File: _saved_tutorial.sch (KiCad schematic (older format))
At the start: 239 parts, among them SW0:0 ESC, SW0:1 1, SW0:10 0, SW0:11 -, SW0:12 =, SW0:13 BCKSPC, SW0:14 INS, SW0:15 HOME, SW0:2 2, SW0:3 3, SW0:4 4, SW0:5 5, SW0:6 6, SW0:7 7, SW0:8 8, SW0:9 9, SW1:0 PAGE_UP, SW1:1 TAB, SW1:10 O, SW1:11 P, SW1:12 [, SW1:13 ], SW1:14 \\, SW1:15 DEL, SW1:2 Q, SW1:3 W, SW1:4 E, SW1:5 R, SW1:6 T, SW1:7 Y, SW1:8 U, SW1:9 I, SW2:0 END, SW2:1 PAGE_DOWN, SW2:10 K, SW2:11 L, SW2:12 ;, SW2:13 `, SW2:14 ENTER, SW2:15 LEFT, SW2:2 CAPSLOCK, SW2:3 A, SW2:4 S, SW2:5 D, SW2:6 F, SW2:7 G, SW2:8 H, SW2:9 J, SW3:0 RIGHT, SW3:1 L_SHIFT, SW3:10 ., SW3:11 /, SW3:12 R_SHIFT, SW3:13 UP, SW3:14 DOWN, SW3:15 L_CTRL, SW3:2 Z, SW3:3 X, SW3:4 C, SW3:5 V, SW3:6 B, SW3:7 N, SW3:8 M, SW3:9 ,, SW4:0 L_SUPER, SW4:1 L_ALT, SW4:10 KEYPAD_1, SW4:11 KEYPAD_2, SW4:12 KEYPAD_3, SW4:13 KEYPAD_4, SW4:14 KEYPAD_5, SW4:15 KEYPAD_6, SW4:2 SPACE, SW4:3 R_ALT, SW4:4 R_SUPER, SW4:5 MENU, SW4:6 R_CTRL, SW4:7 KEYPAD_0, SW4:8 KEYPAD_DEL, SW4:9 KEYPAD_ENTER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

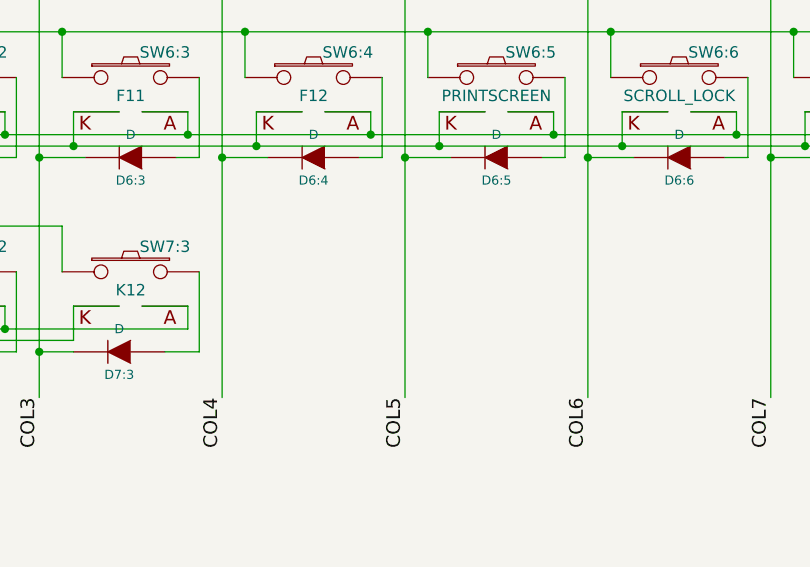
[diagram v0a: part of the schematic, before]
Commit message: first commit
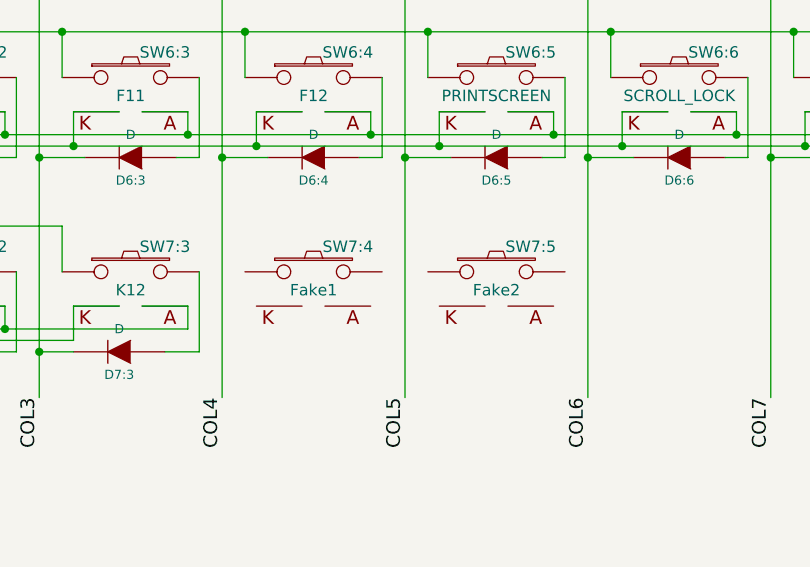
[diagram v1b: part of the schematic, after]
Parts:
- added SW7:4: Fake1, Keyboard:CHERRY_PCB_100H_With_led2, symbol SWITCH_PUSH
- added SW7:5: Fake2, Keyboard:CHERRY_PCB_100H_With_led2, symbol SWITCH_PUSH
- SW0:0, SW0:1, SW0:10, SW0:11, SW0:12, SW0:13, SW0:14, SW0:15, SW0:2, SW0:3, SW0:4, SW0:5, SW0:6, SW0:7, SW0:8, SW0:9, SW1:0, SW1:1, SW1:10, SW1:11, SW1:12, SW1:13, SW1:14, SW1:15, SW1:2, SW1:3, SW1:4, SW1:5, SW1:6, SW1:7, SW1:8, SW1:9, SW2:0, SW2:1, SW2:10, SW2:11, SW2:12, SW2:13, SW2:14, SW2:15, SW2:2, SW2:3, SW2:4, SW2:5, SW2:6, SW2:7, SW2:8, SW2:9, SW3:0, SW3:1, SW3:10, SW3:11, SW3:12, SW3:13, SW3:14, SW3:15, SW3:2, SW3:3, SW3:4, SW3:5, SW3:6, SW3:7, SW3:8, SW3:9, SW4:0, SW4:1, SW4:10, SW4:11, SW4:12, SW4:13, SW4:14, SW4:15, SW4:2, SW4:3, SW4:4, SW4:5, SW4:6, SW4:7, SW4:8, SW4:9, SW5:0, SW5:1, SW5:10, SW5:11, SW5:12, SW5:13, SW5:14, SW5:15, SW5:2, SW5:3, SW5:4, SW5:5, SW5:6, SW5:7, SW5:8, SW5:9, SW6:0, SW6:1, SW6:10, SW6:11, SW6:12, SW6:13, SW6:14, SW6:15, SW6:2, SW6:3, SW6:4, SW6:5, SW6:6, SW6:7, SW6:8, SW6:9, SW7:0, SW7:1, SW7:2, SW7:3: footprint Keyboard:CHERRY_PCB_100H_With_led -> Keyboard:CHERRY_PCB_100H_With_led2

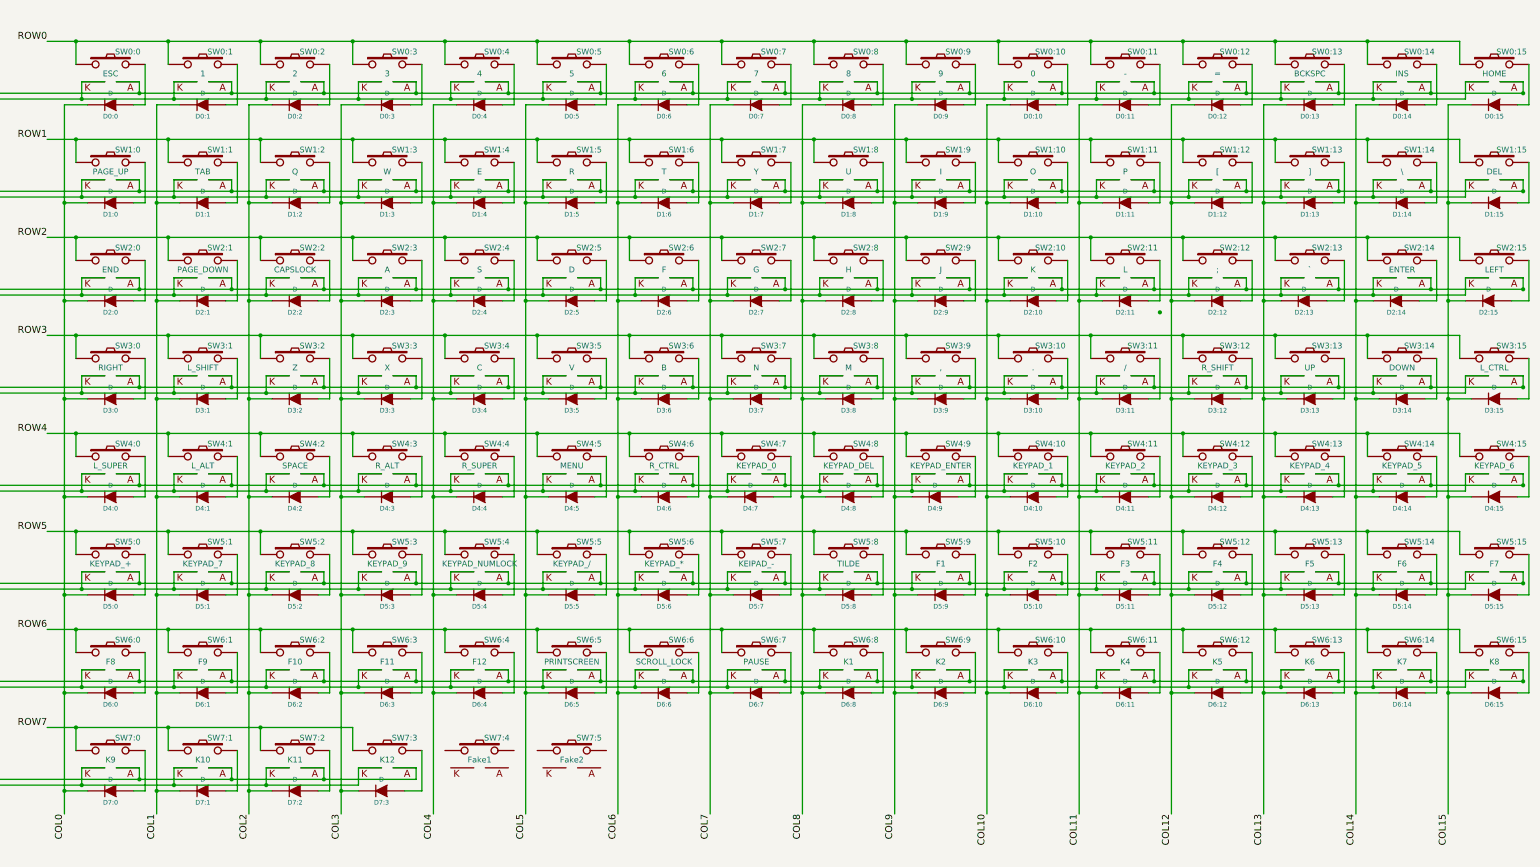
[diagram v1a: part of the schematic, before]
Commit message: another little step
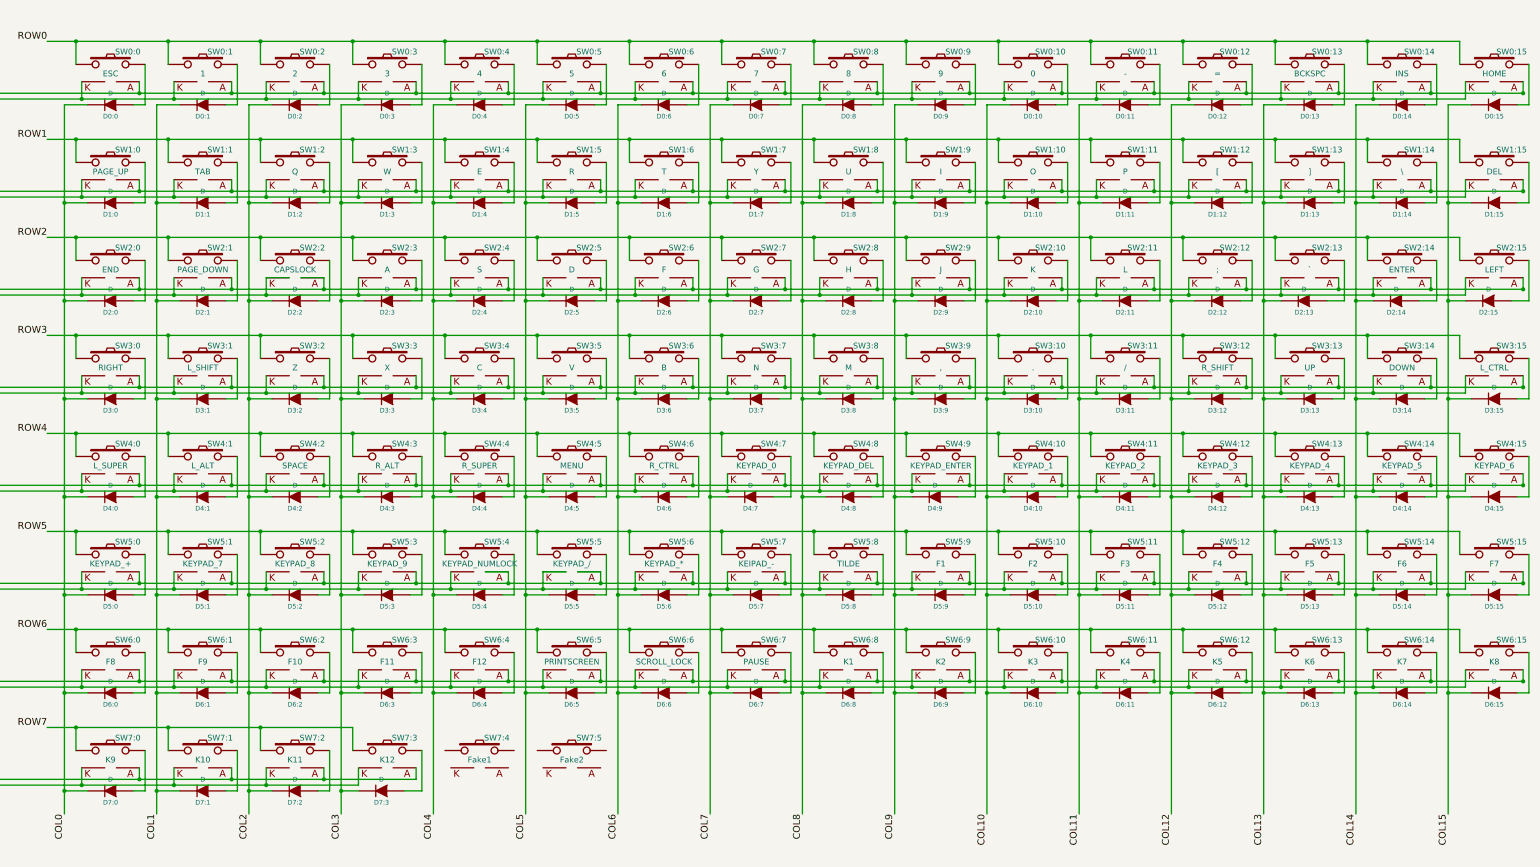
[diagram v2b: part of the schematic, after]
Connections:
- wire segments 972 -> 745
